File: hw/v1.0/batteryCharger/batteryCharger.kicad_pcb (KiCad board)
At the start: 2 copper layers, 40 x 40 mm, 30 parts, among them J1 PWR_IN, J2 USB_B_Micro, J3 USB_C_Receptacle_USB2.0, J4 BAT+, J5 BAT-, U1 LT3652EMSE

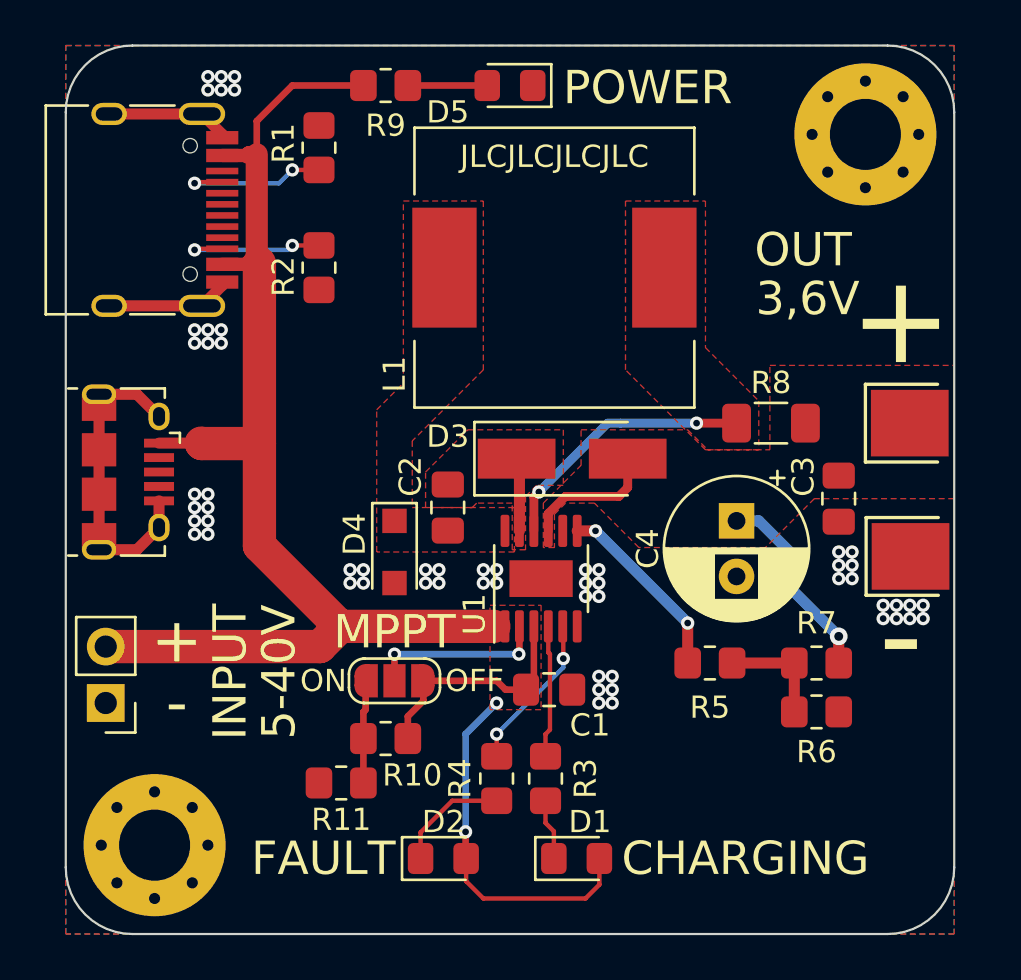
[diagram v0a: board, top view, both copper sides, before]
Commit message: Finished v1.0, mainBoard, batteryCharger
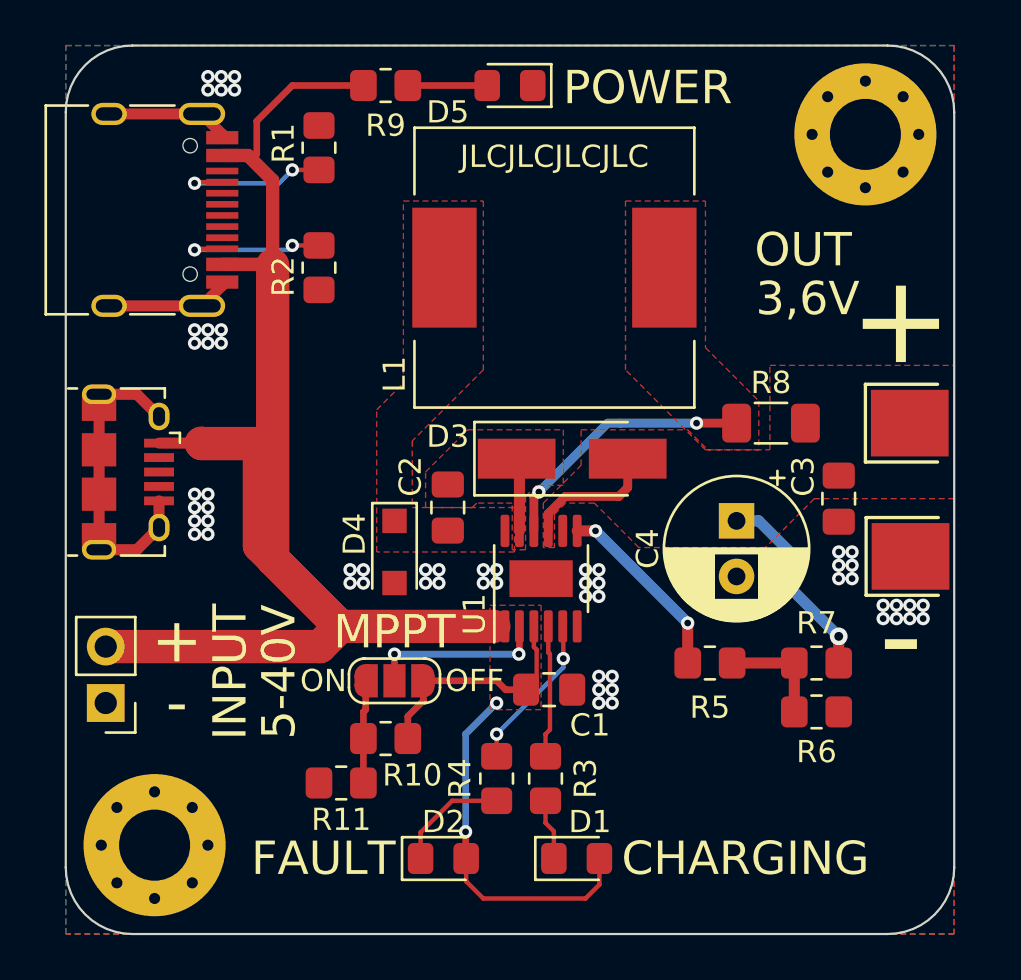
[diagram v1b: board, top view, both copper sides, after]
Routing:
- net VCC: track 82.2 -> 93.1 mm
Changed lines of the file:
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@@
   (net 25 "unconnected-(U1-Pad8)")
   (net 26 "Net-(JP1-Pad1)")
-  (net 27 "Net-(U1-Pad2)")
+  (net 27 "Net-(JP1-Pad2)")
   (footprint "Capacitor_THT:CP_Radial_D6.3mm_P2.50mm" (layer "F.Cu")
     (at 130.2 68.4 -90)
@@
       ))
     (pad "2" smd rect (at 0 0) (size 1 1.5) (layers "F.Cu" "F.Mask")
-      (net 27 "Net-(U1-Pad2)") (pinfunction "C") (pintype "passive"))
+      (net 27 "Net-(JP1-Pad2)") (pinfunction "C") (pintype "passive"))
     (pad "3" smd custom (at 1.3 0) (size 1 0.5) (layers "F.Cu" "F.Mask")
       (net 1 "VCC") (pinfunction "B") (pintype "passive") (zone_connect 2)
@@
       (net 1 "VCC") (pinfunction "VIN") (pintype "power_in"))
     (pad "2" smd roundrect (at -2.15 -0.975 90) (size 1.45 0.4) (layers "F.Cu" "F.Paste" "F.Mask") (roundrect_rratio 0.25)
-      (net 27 "Net-(U1-Pad2)") (pinfunction "VIN_REG") (pintype "input"))
+      (net 27 "Net-(JP1-Pad2)") (pinfunction "VIN_REG") (pintype "input"))
     (pad "3" smd roundrect (at -2.15 -0.325 90) (size 1.45 0.4) (layers "F.Cu" "F.Paste" "F.Mask") (roundrect_rratio 0.25)
       (net 1 "VCC") (pinfunction "~{SHDN}") (pintype "input"))
@@
     (effects (font (size 2 2) (thickness 0.4)))
   )
-  (segment (start 108.20377 51.953544) (end 108.257314 51.9) (width 0.75) (layer "F.Cu") (net 1))
-  (segment (start 107.045 56.85) (end 108.200428 56.85) (width 0.6) (layer "F.Cu") (net 1))
+  (segment (start 121.075 73.15) (end 121.075 74.075) (width 0.2) (layer "F.Cu") (net 1))
   (segment (start 118 83.575) (end 118.025 83.6) (width 0.3) (layer "F.Cu") (net 1))
   (segment (start 112.35 73.15) (end 108.719511 69.519511) (width 1.5) (layer "F.Cu") (net 1))
+  (segment (start 107.045 56.85) (end 109.282924 56.85) (width 0.6) (layer "F.Cu") (net 1))
+  (segment (start 109.282924 56.85) (end 109.316462 56.883538) (width 0.6) (layer "F.Cu") (net 1))
   (segment (start 101.8 74.06) (end 111.44 74.06) (width 1.5) (layer "F.Cu") (net 1))
+  (segment (start 121.075 74.075) (end 121.2 74.2) (width 0.2) (layer "F.Cu") (net 1))
   (segment (start 118.8 85.4) (end 123.4 85.4) (width 0.2) (layer "F.Cu") (net 1))
   (segment (start 113.4 48.8) (end 110.2 48.8) (width 0.3) (layer "F.Cu") (net 1))
-  (segment (start 108.200428 56.85) (end 108.20176 56.851332) (width 0.6) (layer "F.Cu") (net 1))
   (segment (start 116.1 75.6) (end 116.1 76.5) (width 0.3) (layer "F.Cu") (net 1))
-  (segment (start 108.719511 64.919511) (end 108.719511 56.8) (width 1.5) (layer "F.Cu") (net 1))
+  (segment (start 109.316462 53.066236) (end 109.316462 56.883538) (width 0.6) (layer "F.Cu") (net 1))
   (segment (start 121.075 75.65) (end 120.725 76) (width 0.3) (layer "F.Cu") (net 1))
+  (segment (start 108.20377 51.953544) (end 109.316462 53.066236) (width 0.6) (layer "F.Cu") (net 1))
   (segment (start 116.1 76.5) (end 115.4 77.2) (width 0.3) (layer "F.Cu") (net 1))
   (segment (start 118 82.4) (end 118 83.575) (width 0.3) (layer "F.Cu") (net 1))
+  (segment (start 121.2 75.525) (end 120.725 76) (width 0.2) (layer "F.Cu") (net 1))
   (segment (start 108.6 50.4) (end 108.6 51.9) (width 0.3) (layer "F.Cu") (net 1))
   (segment (start 115.4 77.2) (end 115.4 78.2) (width 0.3) (layer "F.Cu") (net 1))
   (segment (start 110.2 48.8) (end 108.6 50.4) (width 0.3) (layer "F.Cu") (net 1))
   (segment (start 108.200226 51.95) (end 108.20377 51.953544) (width 0.6) (layer "F.Cu") (net 1))
+  (segment (start 112.35 73.15) (end 109.316462 70.116462) (width 1.5) (layer "F.Cu") (net 1))
   (segment (start 111.44 74.06) (end 112.35 73.15) (width 1.5) (layer "F.Cu") (net 1))
-  (segment (start 108.20176 56.851332) (end 108.253092 56.8) (width 0.75) (layer "F.Cu") (net 1))
+  (segment (start 109.316462 70.116462) (end 109.316462 56.883538) (width 1.5) (layer "F.Cu") (net 1))
   (segment (start 108.719511 69.519511) (end 108.719511 64.919511) (width 1.5) (layer "F.Cu") (net 1))
   (segment (start 119.4 75.6) (end 119.8 76) (width 0.3) (layer "F.Cu") (net 1))
   (segment (start 106.1 64.9) (end 106.119511 64.919511) (width 1.5) (layer "F.Cu") (net 1))
   (segment (start 123.4 85.4) (end 124.025 84.775) (width 0.2) (layer "F.Cu") (net 1))
+  (segment (start 121.2 74.2) (end 121.2 75.525) (width 0.2) (layer "F.Cu") (net 1))
   (segment (start 116.1 75.6) (end 119.4 75.6) (width 0.3) (layer "F.Cu") (net 1))
   (segment (start 107.045 51.95) (end 108.200226 51.95) (width 0.6) (layer "F.Cu") (net 1))
-  (segment (start 108.6 56.7) (end 108.5 56.8) (width 1) (layer "F.Cu") (net 1))
-  (segment (start 108.257314 51.9) (end 108.6 51.9) (width 0.75) (layer "F.Cu") (net 1))
-  (segment (start 108.253092 56.8) (end 108.5 56.8) (width 0.75) (layer "F.Cu") (net 1))
   (segment (start 118.025 84.625) (end 118.8 85.4) (width 0.2) (layer "F.Cu") (net 1))
-  (segment (start 121.075 73.15) (end 121.075 75.65) (width 0.3) (layer "F.Cu") (net 1))
-  (segment (start 108.6 51.9) (end 108.6 56.7) (width 1) (layer "F.Cu") (net 1))
   (segment (start 118.025 83.6) (end 118.025 84.625) (width 0.2) (layer "F.Cu") (net 1))
   (segment (start 112.35 73.15) (end 119.27548 73.15) (width 1.5) (layer "F.Cu") (net 1))
